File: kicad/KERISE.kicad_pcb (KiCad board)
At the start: 2 copper layers, 40.5 x 38.8 mm, 91 parts, among them J1 Host, J10 Host, J11 Slave, J12 Host, J13 Slave, J14 Motor_L, J15 Motor_R, J2 Slave, J3 Host, J4 Slave, J5 ENC_Host, J6 ENC_Slave, J7 ENC_Host, J8 ENC_Slave, J9 COM, P1 ToF_Host, P2 ToF_Slave, Q1 DMN3065LW-7, Q2 DMN3065LW-7, Q3 SFH3015FA, Q4 DMN3065LW-7, Q5 SFH3015FA, Q6 DMN3065LW-7, Q7 SFH3015FA, Q8 DMN3065LW-7, Q9 SFH3015FA, SW1 RESET, SW2 UPLOAD, U1 ESP32-PICO-D4, U2 VL6180X, U3 PCA9632, U4 ICM-20600, U5 MA730, U6 MA730, U7 LXDC2UR30, U8 DRV8835

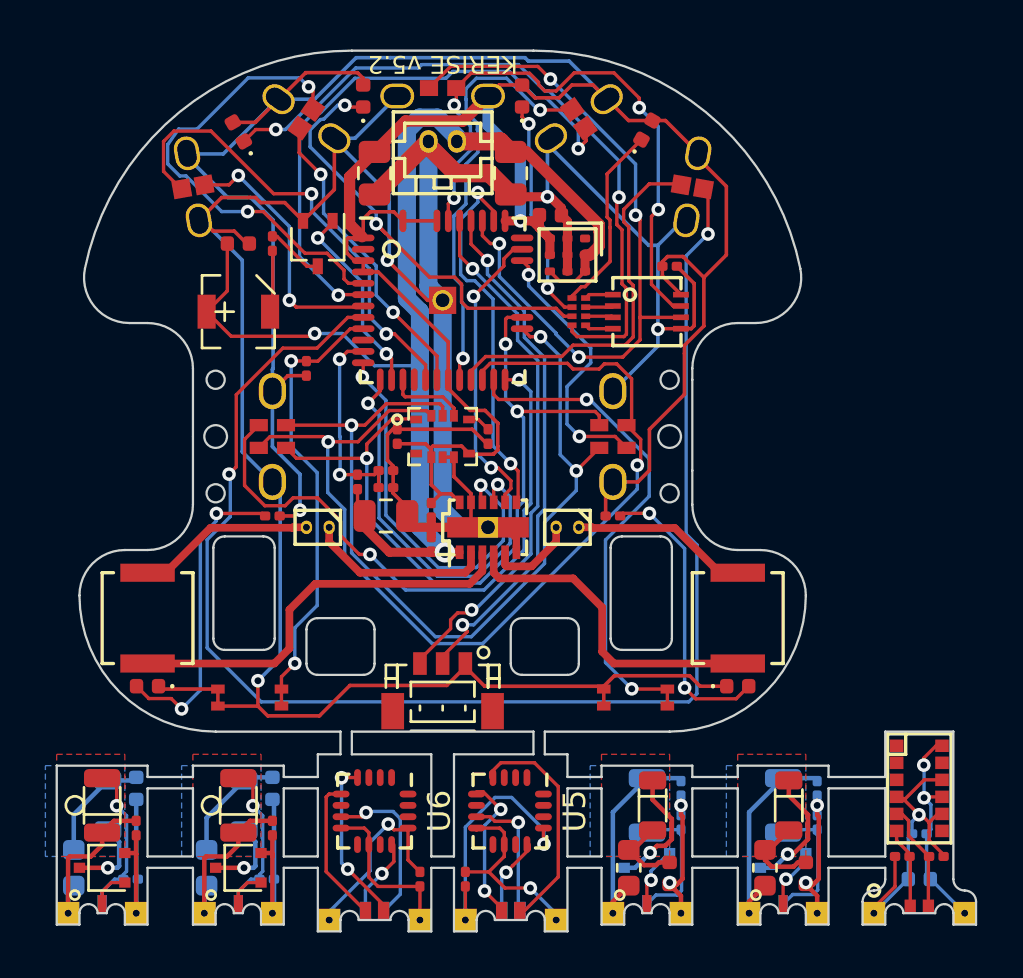
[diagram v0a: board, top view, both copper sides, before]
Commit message: update to kicad 7
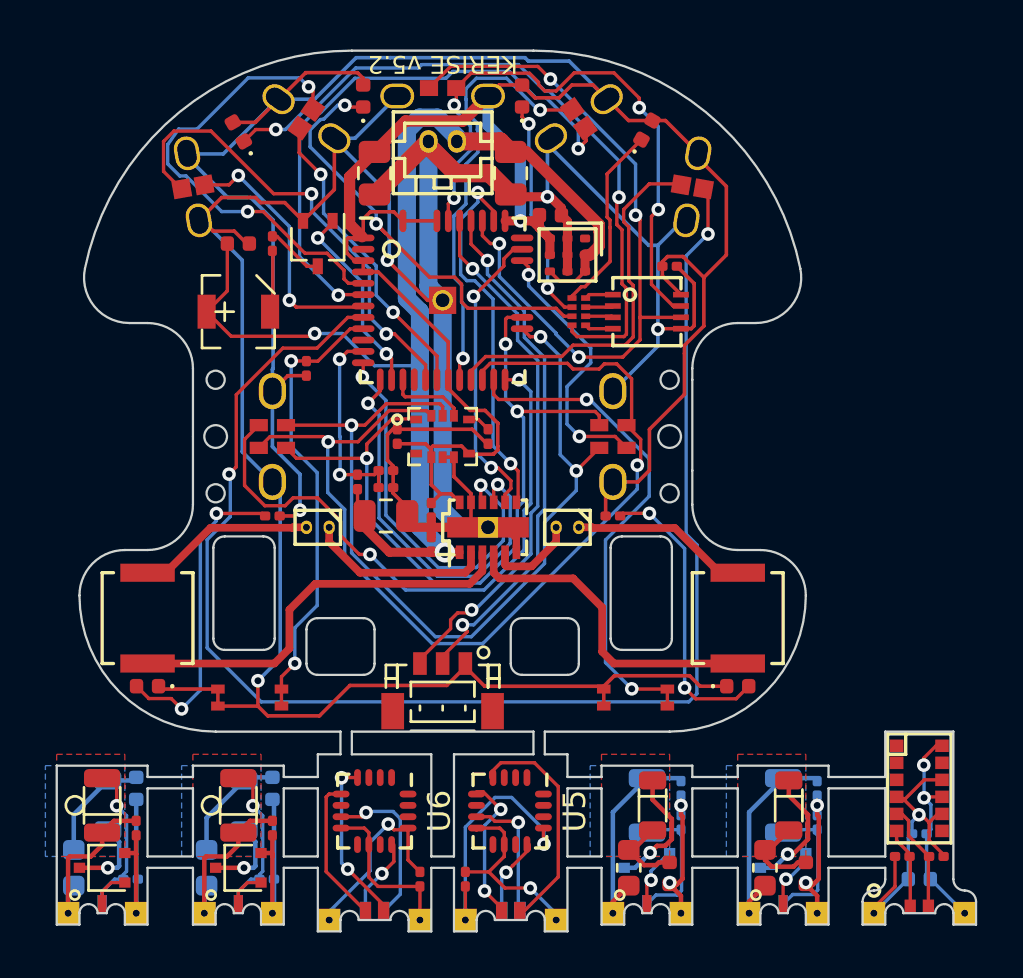
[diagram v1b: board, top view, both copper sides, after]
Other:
- net class 3.3V removed
- net class Analog removed
- net class Antena removed
- net class BATT removed
- net class Default removed
- net class GND removed
- net class LED removed
- net class Motor removed
